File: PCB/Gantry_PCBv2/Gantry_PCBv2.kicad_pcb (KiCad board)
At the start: 2 copper layers, 80 x 90 mm, 206 parts, among them J1 Conn_01x14, J10 Conn_01x05_Female, J11 Conn_01x05_Female, J12 Conn_01x05_Female, J13 B2B-XH-A_LF__SN_, J14 Conn_01x06_Female, J15 Conn_01x07_JST, J16 Conn_01x08_Female, J17 B2B-XH-A_LF__SN_, J18 B2B-XH-A_LF__SN_, J19 Conn_01x04_Female, J2 Conn_01x14, J20 TYPE-C-31-M-12, J3 Conn_01x10, J4 Screw_Terminal_01x02, J5 DCJ200-10-A-XX-X_REVA, J6 Conn_01x03_Male, J7 Conn_01x03_Male, J8 Conn_01x03_Male, J9 Conn_01x03_Male, Q1 SS8050, Q2 SS8050, SW1 SW_Push_DPDT, SW2 SW_Push_DPDT, SW3 SW_Push_Dual, SW4 SW_Push_Dual, SW5 SW_Push_Dual, SW6 SW_Push_Dual, SW7 SW_Push, SW8 SW_Push, U1 ESP32-WROOM-32E, U2 CH340C, U3 TB6612FNG H-bridge Motor Driv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, U4 LM2576, U5 AMS1117

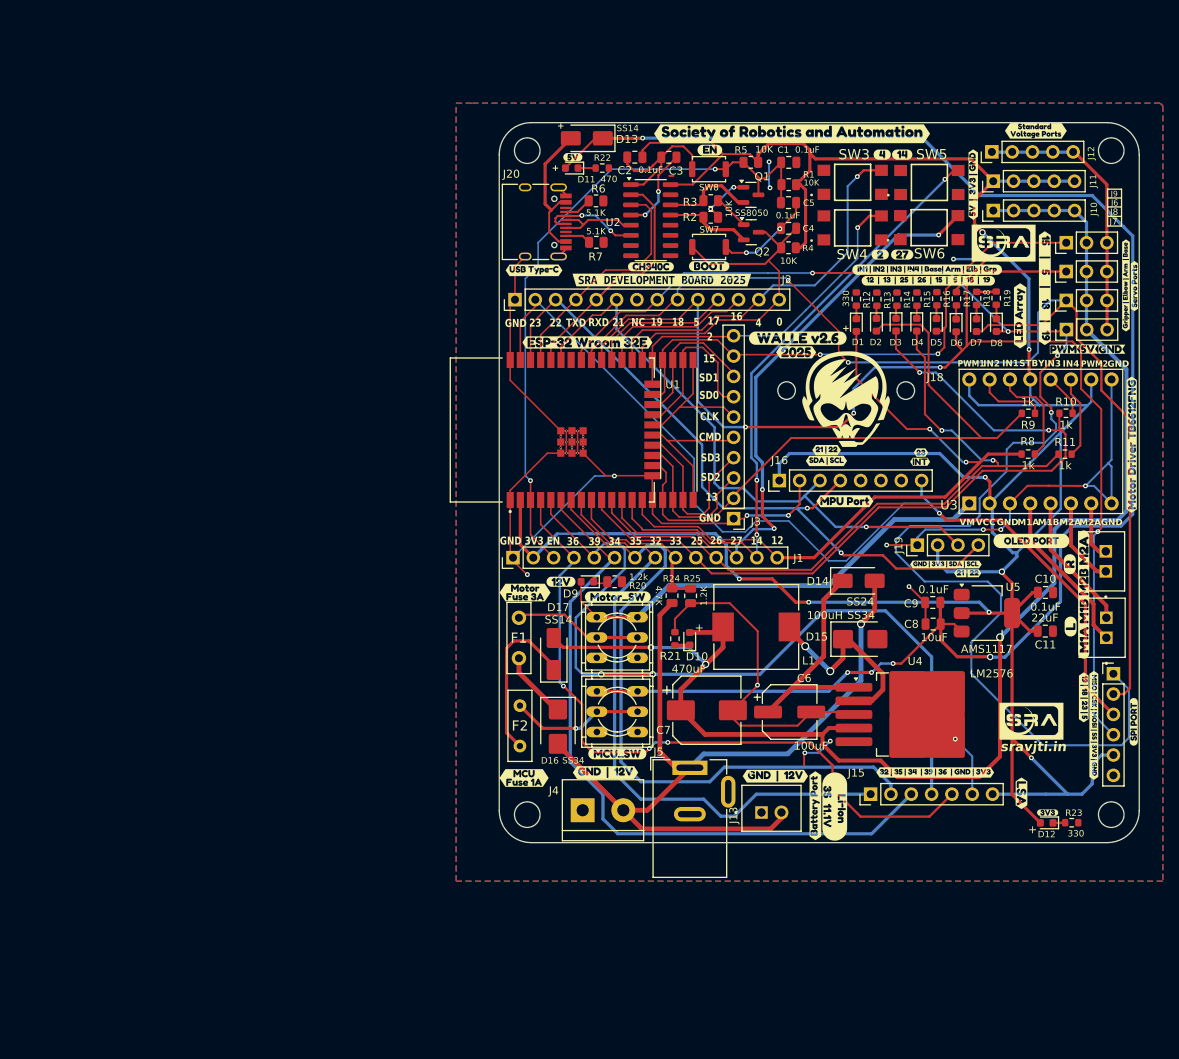
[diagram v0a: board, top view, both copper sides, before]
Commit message: Component Placement done
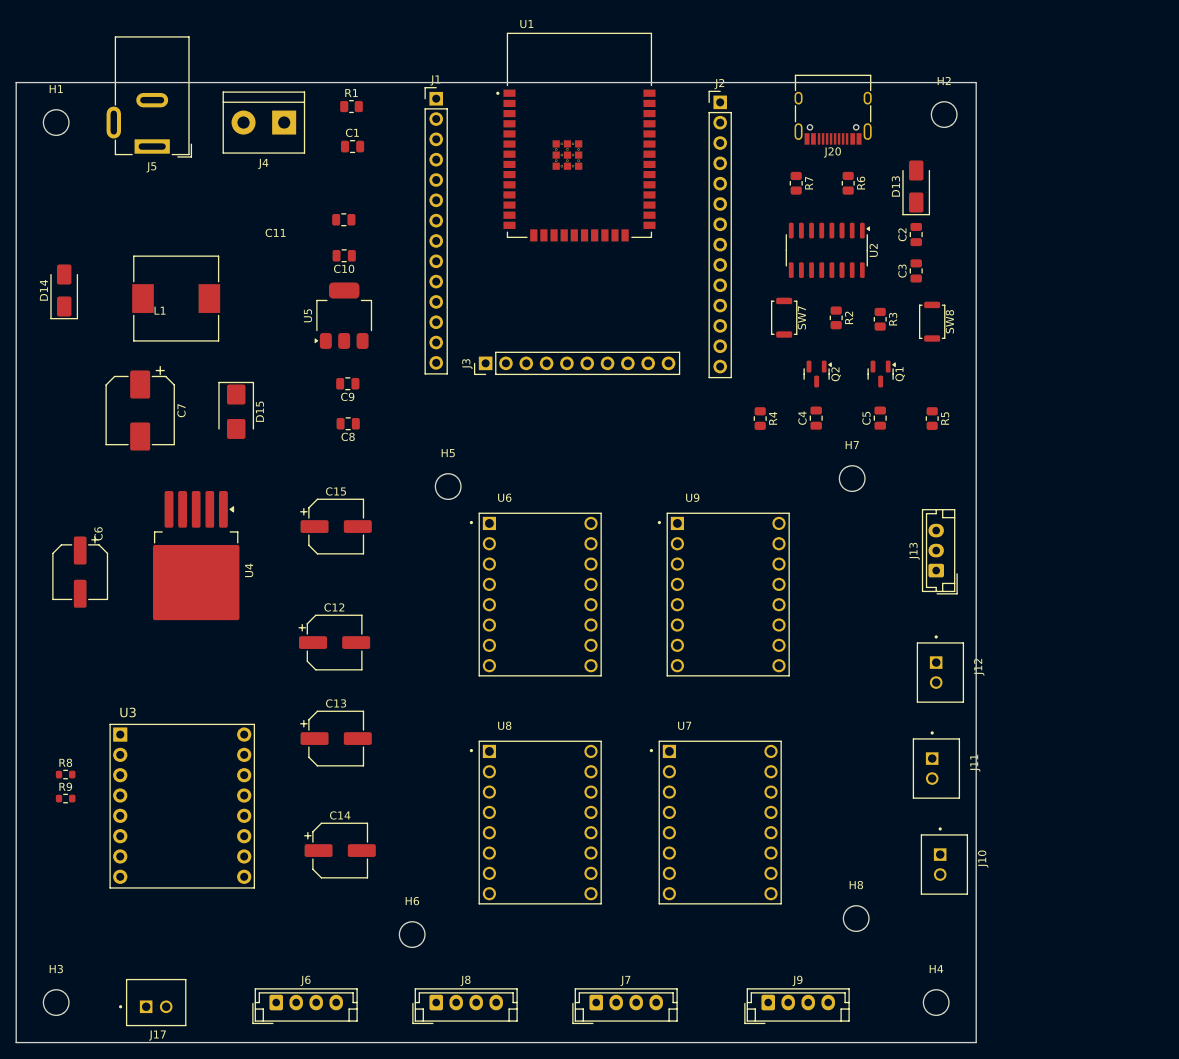
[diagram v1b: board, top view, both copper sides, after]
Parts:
- removed ? (x10): , 
- removed D1, D10, D11, D2, D3, D4, D5, D6, D7, D8, D9: LED, LED_SMD:LED_0603_1608Metric
- removed D12: +, LED_SMD:LED_0603_1608Metric
- removed D16: SS34, Diode_SMD:D_SMB
- removed D17: SS14, Diode_SMD:D_SMA
- removed F1: 3A, PTC Fuse:3A RUEF160
- removed F2: 1A, PTC Fuse:3A RUEF160
- removed G*** (x3): LOGO, logos:sra_logo_small_neg
- removed G***: LOGO, logos:espressif_logo
- removed G*** (x2): LOGO, logos:sra_skull_big
- removed G***: LOGO, logos:sra_board_github_qr_code
- removed G***: LOGO, Logos:Lions_logo
- removed G***: LOGO, Logos:kicad_logo
- removed G***: LOGO, Logos:sra_logo_big
- removed J14: Conn_01x06_Female, Connector_PinHeader_2.54mm:PinHeader_1x06_P2.54mm_Vertical
- removed J15: Conn_01x07_JST, Connector_PinHeader_2.54mm:PinHeader_1x07_P2.54mm_Vertical
- removed J16: Conn_01x08_Female, Connector_PinHeader_2.54mm:PinHeader_1x08_P2.54mm_Vertical
- removed J18: B2B-XH-A_LF__SN_, JST Connector:2 Pin JST Connector
- removed J19: Conn_01x04_Female, Connector_PinHeader_2.54mm:PinHeader_1x04_P2.54mm_Vertical
- removed R10, R11: 1k, Resistor_SMD:R_0603_1608Metric
- removed R12, R13, R14, R15, R16, R17, R18, R19, R23: 330, Resistor_SMD:R_0603_1608Metric
- removed R20: 1.2k, Resistor_SMD:R_0805_2012Metric
- removed R21, R22: 470, Resistor_SMD:R_0603_1608Metric
- removed R24: 4.7K, Resistor_SMD:R_0805_2012Metric
- removed R25: 1.2K, Resistor_SMD:R_0805_2012Metric
- removed REF** (x2): MountingHole_2.2mm_M2, MountingHole:MountingHole_2.2mm_M2
- removed SW1, SW2: SW_Push_DPDT, Switches:dpdt_sw_2x03_tht
- removed SW3, SW4, SW5, SW6: SW_Push_Dual, Switches:spst_tactile_sw_2x02_smd
- removed kibuzzard-658F2C13 (x2): G***, kibuzzard-658F2C13
- removed kibuzzard-658F2C3C (x2): G***, kibuzzard-658F2C3C
- removed kibuzzard-668D4F46 (x2): G***, kibuzzard-668D4F46
- removed kibuzzard-668D4F81 (x2): G***, kibuzzard-668D4F81
- removed kibuzzard-668D5592: G***, kibuzzard-668D5592
- removed kibuzzard-668D6178: G***, kibuzzard-668D6178
- removed kibuzzard-668FE423: G***, kibuzzard-668FE423
- removed kibuzzard-668FF9B2 (x2): G***, kibuzzard-668FF9B2
- removed kibuzzard-66914CE9: G***, kibuzzard-66914CE9
- removed kibuzzard-669207B4: G***, kibuzzard-669207B4
- removed kibuzzard-66920921: G***, kibuzzard-66920921
- removed kibuzzard-6692092C: G***, kibuzzard-6692092C
- removed kibuzzard-66920939: G***, kibuzzard-66920939
- removed kibuzzard-66921043: G***, kibuzzard-66921043
- removed kibuzzard-66923428: G***, kibuzzard-66923428
- removed kibuzzard-66CD8CDE: G***, kibuzzard-66CD8CDE
- removed kibuzzard-66CD901B: G***, kibuzzard-66CD901B
- removed kibuzzard-66CD90B0 (x2): G***, kibuzzard-66CD90B0
- removed kibuzzard-66CDCB66: G***, kibuzzard-66CDCB66
- removed kibuzzard-66CDD771: G***, kibuzzard-66CDD771
- removed kibuzzard-66CDD792 (x2): G***, kibuzzard-66CDD792
- removed kibuzzard-66CDD7A1 (x2): G***, kibuzzard-66CDD7A1
- removed kibuzzard-66CDD7D8 (x2): G***, kibuzzard-66CDD7D8
- removed kibuzzard-66CF838C (x2): G***, kibuzzard-66CF838C
- removed kibuzzard-66CF83B9 (x2): G***, kibuzzard-66CF83B9
- removed kibuzzard-66CF86D1 (x2): G***, kibuzzard-66CF86D1
- removed kibuzzard-66CF86E5 (x2): G***, kibuzzard-66CF86E5
- removed kibuzzard-66D06403: G***, kibuzzard-66D06403
- removed kibuzzard-66D06F4C: G***, kibuzzard-66D06F4C
- removed kibuzzard-66D06F54: G***, kibuzzard-66D06F54
- removed kibuzzard-66D0BB59: G***, kibuzzard-66D0BB59
- removed kibuzzard-66D58886: G***, kibuzzard-66D58886
- removed kibuzzard-675FD791: G***, kibuzzard-675FD791
- removed kibuzzard-675FDA6A: G***, kibuzzard-675FDA6A
- removed kibuzzard-675FDACE: G***, kibuzzard-675FDACE
- removed kibuzzard-675FDAD6: G***, kibuzzard-675FDAD6
- removed kibuzzard-675FDAE3: G***, kibuzzard-675FDAE3
- removed kibuzzard-675FDAEB: G***, kibuzzard-675FDAEB
- removed kibuzzard-675FDD5C: G***, kibuzzard-675FDD5C
- removed kibuzzard-675FDE17: G***, kibuzzard-675FDE17
- removed kibuzzard-675FE5A8: G***, kibuzzard-675FE5A8
- removed kibuzzard-675FE5B2: G***, kibuzzard-675FE5B2
- removed kibuzzard-675FEDA3: G***, kibuzzard-675FEDA3
- removed kibuzzard-675FF2F7: G***, kibuzzard-675FF2F7
- removed kibuzzard-675FF2FE (x2): G***, kibuzzard-675FF2FE
- removed kibuzzard-675FF39E: G***, kibuzzard-675FF39E
- removed kibuzzard-675FF567: G***, kibuzzard-675FF567
- removed kibuzzard-675FF648: G***, kibuzzard-675FF648
- removed kibuzzard-67602BF7: G***, kibuzzard-67602BF7
- removed kibuzzard-67602C07: G***, kibuzzard-67602C07
- removed kibuzzard-67602C35: G***, kibuzzard-67602C35
- removed kibuzzard-67602C64: G***, kibuzzard-67602C64
- removed kibuzzard-67602CD0: G***, kibuzzard-67602CD0
- removed kibuzzard-67602CEF: G***, kibuzzard-67602CEF
- removed kibuzzard-67602E60: G***, kibuzzard-67602E60
- removed kibuzzard-67602E69: G***, kibuzzard-67602E69
- removed kibuzzard-67602EA4: G***, kibuzzard-67602EA4
- removed kibuzzard-67704BF1: G***, kibuzzard-67704BF1
- removed kibuzzard-67704C04: G***, kibuzzard-67704C04
- removed kibuzzard-67704CCE: G***, kibuzzard-67704CCE
- removed kibuzzard-67704CDF: G***, kibuzzard-67704CDF
- removed kibuzzard-67704CF4: G***, kibuzzard-67704CF4
- removed kibuzzard-67704D11: G***, kibuzzard-67704D11
- removed kibuzzard-67704D22: G***, kibuzzard-67704D22
- removed kibuzzard-67704D9C: G***, kibuzzard-67704D9C
- removed kibuzzard-677158DD: G***, kibuzzard-677158DD
- removed kibuzzard-67715A02: G***, kibuzzard-67715A02
- removed kibuzzard-67715A46: G***, kibuzzard-67715A46
- removed kibuzzard-6774F3BB: G***, kibuzzard-6774F3BB
- removed kibuzzard-6774F4AA: G***, kibuzzard-6774F4AA
- removed kibuzzard-6774F4AE: G***, kibuzzard-6774F4AE
- removed kibuzzard-6774F51E: G***, kibuzzard-6774F51E
- removed kibuzzard-67A02922: G***, kibuzzard-67A02922
- removed kibuzzard-67BF910C: G***, kibuzzard-67BF910C
- removed kibuzzard-67BF911E: G***, kibuzzard-67BF911E
- added C12: 100u, Capacitor_SMD:CP_Elec_6.3x7.7, F.Cu at (89.8, 120.0)
- added C13: 100u, Capacitor_SMD:CP_Elec_6.3x7.7, F.Cu at (90.0, 132.0)
- added C14: 100u, Capacitor_SMD:CP_Elec_6.3x7.7, F.Cu at (90.5, 146.0)
- added C15: 100u, Capacitor_SMD:CP_Elec_6.3x7.7, F.Cu at (90.0, 105.5)
- added H5: MountingHole, MountingHole:MountingHole_3.2mm_M3, F.Cu at (104.0, 100.5)
- added H6: MountingHole, MountingHole:MountingHole_3.2mm_M3, F.Cu at (99.5, 156.5)
- added H7: MountingHole, MountingHole:MountingHole_3.2mm_M3, F.Cu at (154.5, 99.5)
- added H8: MountingHole, MountingHole:MountingHole_3.2mm_M3, F.Cu at (155.0, 154.5)
- added U6: DRV8825_STEPPER_MOTOR_DRIVER_CARRIER, DRV8825_STEPPER_MOTOR_DRIVER_CARRIER (1):IC_DRV8825_STEPPER_MOTOR_DRIVER_CARRIER, F.Cu at (115.5, 114.0)
- added U7: DRV8825_STEPPER_MOTOR_DRIVER_CARRIER, DRV8825_STEPPER_MOTOR_DRIVER_CARRIER (1):IC_DRV8825_STEPPER_MOTOR_DRIVER_CARRIER, F.Cu at (138.0, 142.5)
- added U8: DRV8825_STEPPER_MOTOR_DRIVER_CARRIER, DRV8825_STEPPER_MOTOR_DRIVER_CARRIER (1):IC_DRV8825_STEPPER_MOTOR_DRIVER_CARRIER, F.Cu at (115.5, 142.5)
- added U9: DRV8825_STEPPER_MOTOR_DRIVER_CARRIER, DRV8825_STEPPER_MOTOR_DRIVER_CARRIER (1):IC_DRV8825_STEPPER_MOTOR_DRIVER_CARRIER, F.Cu at (139.0, 114.0)
- J10, J11, J12: value Conn_01x05_Female -> B2B-XH-A_LF__SN_; footprint Connector_PinHeader_2.54mm:PinHeader_1x05_P2.54mm_Vertical -> 2 Pin JST_Power&Motors:JST_B2B-XH-A_LF__SN_
- J13: value B2B-XH-A_LF__SN_ -> Conn_01x03_Pin; footprint JST Connector:2 Pin JST Connector -> Connector_JST:JST_EH_B3B-EH-A_1x03_P2.50mm_Vertical
- J17: footprint JST Connector:2 Pin JST Connector -> 2 Pin JST_Power&Motors:JST_B2B-XH-A_LF__SN_
- J6, J7, J8, J9: value Conn_01x03_Male -> Conn_01x04_Pin; footprint Connector_PinHeader_2.54mm:PinHeader_1x03_P2.54mm_Vertical -> Connector_JST:JST_EH_B4B-EH-A_1x04_P2.50mm_Vertical
- SW7: value SW_Push -> SW_0
- SW8: value SW_Push -> SW_EN
- U1: footprint ESP-32:ESP32-WROOM-32E__4MB_HIGH_TEMP_ -> ESP32-WROOM:XCVR_ESP32-WROOM-32E__4MB_HIGH_TEMP_
- U3: footprint Motor Drivers:TB6612FNG -> motor_driver:TB6612FNG
- U4: value LM2576 -> LM2576S-5
- U5: value AMS1117 -> AMS1117-3.3
- moved J6 134.5 mm to (82.5, 165.0), turned to 0 degrees
- moved H3 134.0 mm to (55.0, 165.0)
- moved R9 129.6 mm to (56.2, 139.5)
- moved J17 127.2 mm to (67.5, 165.0), turned to 0 degrees
- moved R8 126.8 mm to (56.2, 136.5)
- moved J8 117.9 mm to (102.5, 165.0), turned to 0 degrees
- moved U3 113.3 mm to (70.6, 137.8), turned to 0 degrees
- moved H4 108.7 mm to (165.0, 165.0)
- moved D14 105.7 mm to (56.0, 76.0), turned to 90 degrees
- moved J5 102.7 mm to (67.0, 58.0), turned to 180 degrees
- moved J7 102.6 mm to (122.5, 165.0), turned to 0 degrees
- moved J9 102.0 mm to (144.0, 165.0), turned to 0 degrees
- moved H2 101.9 mm to (166.0, 54.0)
- moved C11 101.7 mm to (91.0, 67.2), turned to 180 degrees
- moved C10 97.2 mm to (91.0, 71.7), turned to 180 degrees
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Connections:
- J10 pad 1: /5V -> /15
- J10 pad 2: /5V -> GND
- J11 pad 1: /3V3 -> /19
- J11 pad 2: /3V3 -> GND
- J12 pad 1: GND -> /18
- J13 pad 1: GND -> unconnected-(J13-Pin_1-Pad1)
- J13 pad 2: /12V -> /12V_P
- J20 pad A1: GND -> (no net)
- J20 pad A12: GND -> (no net)
- J20 pad A4: /VBUSC -> (no net)
- J20 pad A9: /VBUSC -> (no net)
- J20 pad B1: GND -> (no net)
- J20 pad B12: GND -> (no net)
- J20 pad B4: /VBUSC -> (no net)
- J20 pad B9: /VBUSC -> (no net)
- J6 pad 1: /5 -> /SM2_A1
- J6 pad 2: /5V -> /SM2_A2
- J6 pad 3: GND -> /SM2_B1
- J7 pad 1: /19 -> /SM3_A1
- J7 pad 2: /5V -> /SM3_A2
- J7 pad 3: GND -> /SM3_B1
- J8 pad 1: /18 -> /SM4_A1
- J8 pad 2: /5V -> /SM4_A2
- J8 pad 3: GND -> /SM4_B1
- J9 pad 1: /15 -> /SM1_A1
- J9 pad 2: /5V -> /SM1_A2
- J9 pad 3: GND -> /SM1_B1
- R8 pad 1: /12 -> /18
- U1 pad 17: /SD2 -> unconnected-(U1-NC-Pad17)
- U1 pad 18: /SD3 -> unconnected-(U1-NC-Pad18)
- U1 pad 19: /CMD -> unconnected-(U1-NC-Pad19)
- U1 pad 20: /CLK -> unconnected-(U1-NC-Pad20)
- U1 pad 21: /SD0 -> unconnected-(U1-NC-Pad21)
- U1 pad 22: /SD1 -> unconnected-(U1-NC-Pad22)
- U1 pad 39_1: GND -> (no net)
- U1 pad 39_10: GND -> (no net)
- U1 pad 39_11: GND -> (no net)
- U1 pad 39_12: GND -> (no net)
- U1 pad 39_13: GND -> (no net)
- U1 pad 39_14: GND -> (no net)
- U1 pad 39_15: GND -> (no net)
- U1 pad 39_16: GND -> (no net)
- U1 pad 39_17: GND -> (no net)
- U1 pad 39_18: GND -> (no net)
- U1 pad 39_19: GND -> (no net)
- U1 pad 39_2: GND -> (no net)
- U1 pad 39_20: GND -> (no net)
- U1 pad 39_21: GND -> (no net)
- U1 pad 39_3: GND -> (no net)
- U1 pad 39_4: GND -> (no net)
- U1 pad 39_5: GND -> (no net)
- U1 pad 39_6: GND -> (no net)
- U1 pad 39_7: GND -> (no net)
- U1 pad 39_8: GND -> (no net)
- U1 pad 39_9: GND -> (no net)
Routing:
- net /3V3: track 378.3 -> 0.06 mm, vias 8 -> 0
- net GND: track 321.1 -> 0.00 mm, vias 19 -> 0
- net /5V_P: track 203.6 -> 0.00 mm, vias 5 -> 0
- net /5V: track 178.5 -> 0.00 mm, vias 3 -> 0
- net /19: track 174.9 -> 0.00 mm, vias 5 -> 0
- net /5: track 158.9 -> 0.00 mm, vias 4 -> 0
- net /18: track 144.2 -> 0.00 mm, vias 2 -> 0
- net /23: track 122.2 -> 0.00 mm, vias 1 -> 0
- net /12V: track 107.1 -> 0.00 mm, vias 1 -> 0
- net /25: track 102.0 -> 0.00 mm, vias 2 -> 0
- net /39: track 99.7 -> 0.00 mm, vias 2 -> 0
- net /26: track 89.3 -> 0.59 mm, vias 2 -> 0
- net /34: track 88.4 -> 0.00 mm
- net /36: track 87.6 -> 0.00 mm, vias 3 -> 0
- net /22: track 86.9 -> 0.00 mm, vias 2 -> 0
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- removed copper zone on B.Cu, net GND
- removed copper zone on F.Cu, net GND
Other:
- board size 80 x 90 mm -> 120 x 120 mm
- board text removed: "+"
- board text removed: "0"
- board text removed: "12"
- board text removed: "13"
- board text removed: "14"
- board text removed: "15"
- board text removed: "16"
- board text removed: "17"
- board text removed: "18"
- board text removed: "19"
- board text removed: "2"
- board text removed: "21"
- board text removed: "22"
- board text removed: "23"
- board text removed: "25"
- board text removed: "26"
- board text removed: "27"
- board text removed: "32"
- board text removed: "33"
- board text removed: "34"
- board text removed: "35"
- board text removed: "36"
- board text removed: "39"
- board text removed: "3V3 GND"
- board text removed: "4"
- board text removed: "5"
- board text removed: "CLK"
- board text removed: "CMD"
- board text removed: "Designed by"
- board text removed: "EN"
- board text removed: "GND"
- board text removed: "GND 3V3"
- board text removed: "IN1"
- board text removed: "IN2"
- board text removed: "IN3"
- board text removed: "IN4"
- board text removed: "M1A"
- board text removed: "M1B"
- board text removed: "M2A"
- board text removed: "NC"
- board text removed: "PWM1"
- board text removed: "PWM2"
- board text removed: "RXD"
- board text removed: "SD0"
- board text removed: "SD1"
- board text removed: "SD2"
- board text removed: "SD3"
- board text removed: "STBY"
- board text removed: "TXD"
- board text removed: "VCC"
- board text removed: "VM"
- board text removed: "sravjti.in"
